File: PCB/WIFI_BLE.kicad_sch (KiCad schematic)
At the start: 25 parts, among them J901 73412-0110, U901 LBEE5PK2AE-771

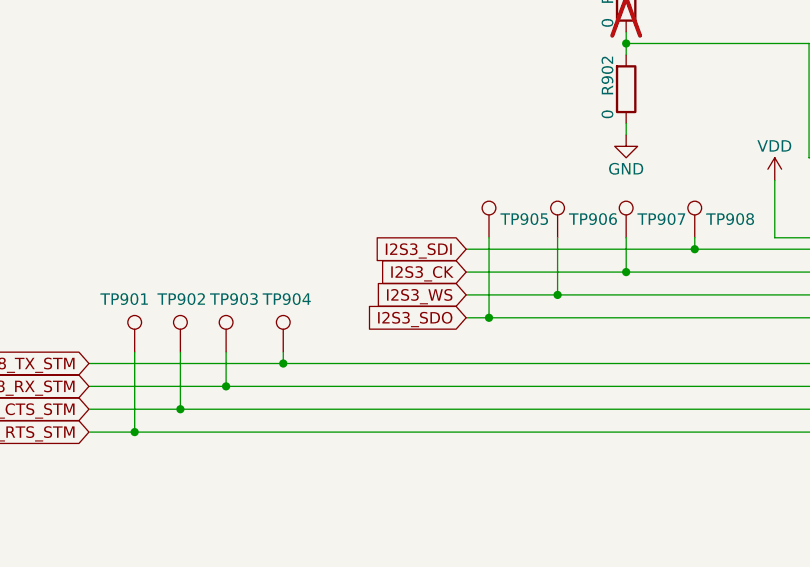
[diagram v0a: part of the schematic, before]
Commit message: pcb_update
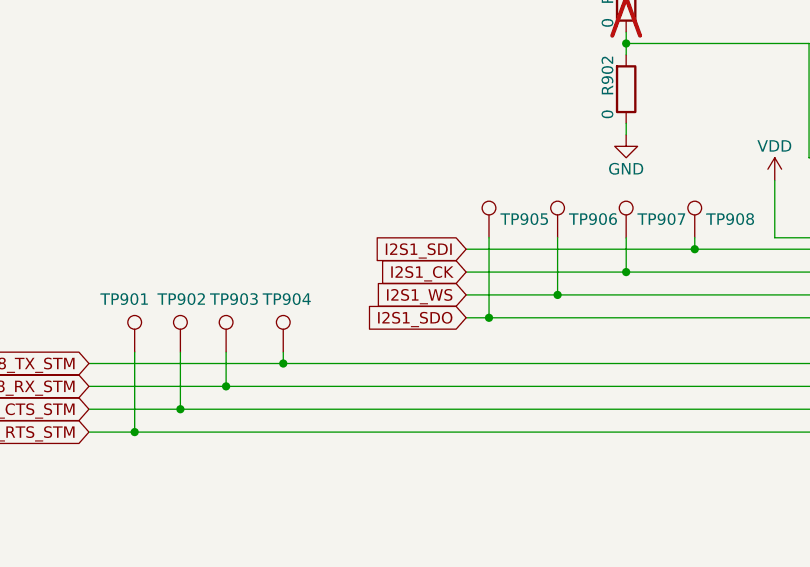
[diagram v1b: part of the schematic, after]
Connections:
- net I2S3_CK renamed I2S1_CK
- net I2S3_SDI renamed I2S1_SDI
- net I2S3_SDO renamed I2S1_SDO
- net I2S3_WS renamed I2S1_WS
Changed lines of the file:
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@@
 		)
 	)
-	(global_label "I2S3_WS"
+	(global_label "I2S1_WS"
 		(shape input)
 		(at 91.44 124.46 180)
@@
 		)
 	)
-	(global_label "I2S3_SDO"
+	(global_label "I2S1_SDO"
 		(shape input)
 		(at 91.44 127 180)
@@
 		)
 	)
-	(global_label "I2S3_SDI"
+	(global_label "I2S1_SDI"
 		(shape input)
 		(at 91.44 119.38 180)
@@
 		)
 	)
-	(global_label "I2S3_CK"
+	(global_label "I2S1_CK"
 		(shape input)
 		(at 91.44 121.92 180)

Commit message: PCB_UPDATE
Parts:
- TP901, TP902, TP903, TP904, TP905, TP906, TP907, TP908: footprint TestPoint:TestPoint_Pad_D1.0mm -> Library:TP_0.5mm
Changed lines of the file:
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@@
 		)
 	)
+	(rule_area
+		(polyline
+			(pts
+				(xy 406.4 12.7) (xy 406.4 251.46) (xy 298.45 251.46) (xy 298.45 284.48) (xy 12.7 284.48) (xy 12.7 12.7)
+			)
+			(stroke
+				(width 0)
+				(type dash)
+			)
+			(fill
+				(type none)
+			)
+		)
+	)
+	(netclass_flag ""
+		(length 2.54)
+		(shape round)
+		(at 27.94 12.7 180)
+		(fields_autoplaced yes)
+		(effects
+			(font
+				(size 1.27 1.27)
+			)
+			(justify right bottom)
+		)
+		(property "Netclass" "WIFI_BLE"
+			(at 28.6385 15.24 0)
+			(effects
+				(font
+					(size 1.27 1.27)
+				)
+				(justify left)
+			)
+		)
+		(property "Component Class" ""
+			(at -124.46 7.62 0)
+			(effects
+				(font
+					(size 1.27 1.27)
+					(italic yes)
+				)
+			)
+		)
+	)
 	(symbol
 		(lib_id "power:+36V")
@@
 			)
 		)
-		(property "Footprint" "TestPoint:TestPoint_Pad_D1.0mm"
+		(property "Footprint" "Library:TP_0.5mm"
 			(at 59.69 130.81 0)
 			(effects
@@
 			)
 		)
-		(property "Footprint" "TestPoint:TestPoint_Pad_D1.0mm"
+		(property "Footprint" "Library:TP_0.5mm"
 			(at 106.68 118.11 0)
 			(effects
@@
 			)
 		)
-		(property "Footprint" "TestPoint:TestPoint_Pad_D1.0mm"
+		(property "Footprint" "Library:TP_0.5mm"
 			(at 114.3 118.11 0)
 			(effects
@@
 			)
 		)
-		(property "Footprint" "TestPoint:TestPoint_Pad_D1.0mm"
+		(property "Footprint" "Library:TP_0.5mm"
 			(at 76.2 130.81 0)
 			(effects
@@
 			)
 		)
-		(property "Footprint" "TestPoint:TestPoint_Pad_D1.0mm"
+		(property "Footprint" "Library:TP_0.5mm"
 			(at 69.85 130.81 0)
 			(effects
@@
 			)
 		)
-		(property "Footprint" "TestPoint:TestPoint_Pad_D1.0mm"
+		(property "Footprint" "Library:TP_0.5mm"
 			(at 99.06 118.11 0)
 			(effects
@@
 			)
 		)
-		(property "Footprint" "TestPoint:TestPoint_Pad_D1.0mm"
+		(property "Footprint" "Library:TP_0.5mm"
 			(at 121.92 118.11 0)
 			(effects
@@
 			)
 		)
-		(property "Footprint" "TestPoint:TestPoint_Pad_D1.0mm"
+		(property "Footprint" "Library:TP_0.5mm"
 			(at 64.77 130.81 0)
 			(effects
